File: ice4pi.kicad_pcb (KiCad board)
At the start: 4 copper layers, 65 x 30 mm, 66 parts, among them J1 Pmod 2x6, J2 Raspberry_Pi_2_3, U1 ICE40HX1K-TQ144, U2 W25Q32JVSSIQ(SOIC-8_208mil), U3 LT3030, U4 DSC1001DI1-012.0000, U5 TFDU4101-TR3

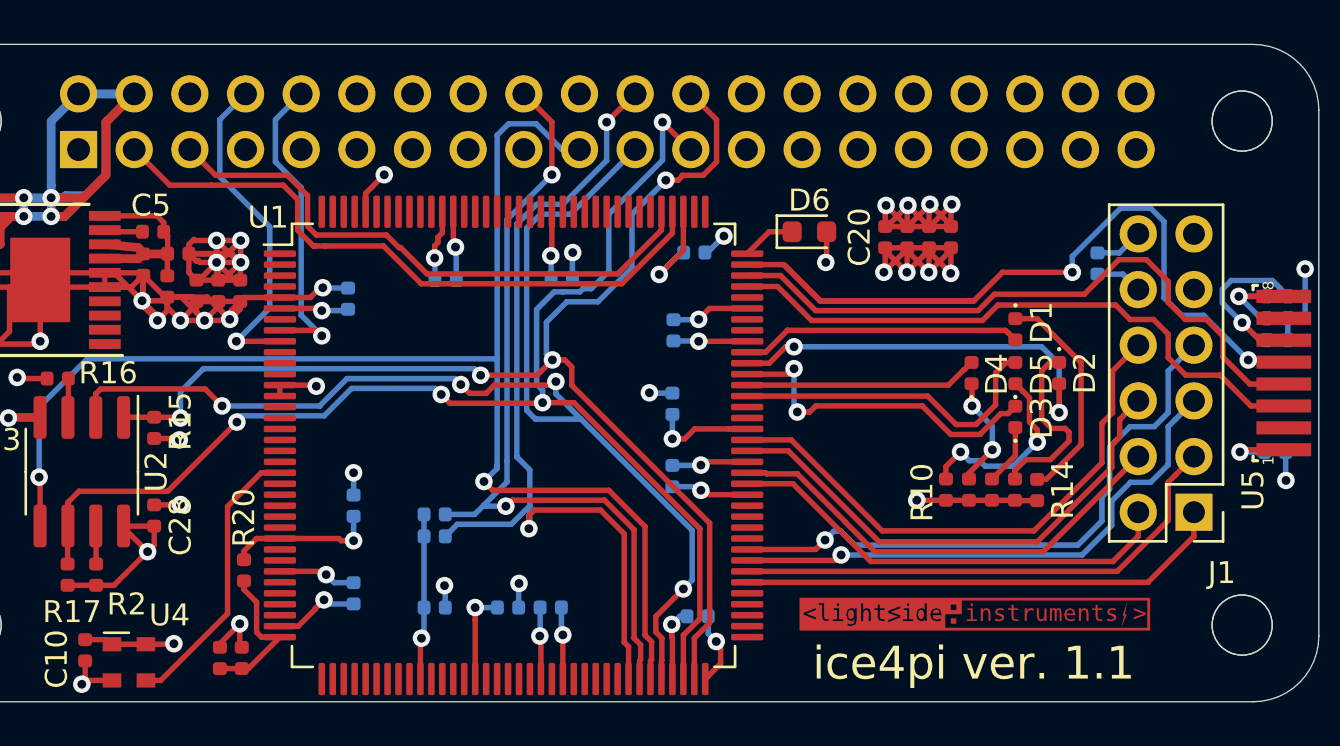
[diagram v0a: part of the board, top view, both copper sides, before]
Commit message: Release 1.2
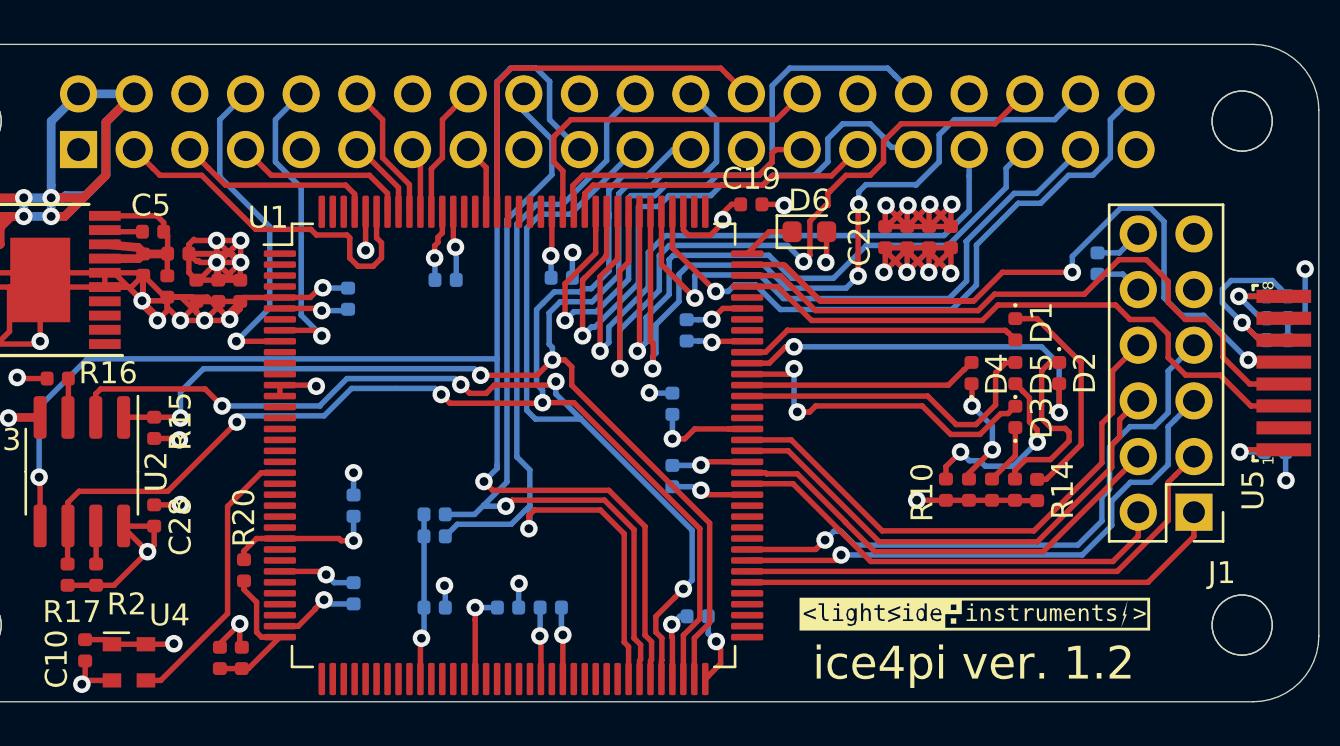
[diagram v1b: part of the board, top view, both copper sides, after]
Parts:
- C19: moved to F.Cu
- U2: value W25Q32JVSSIQ(SOIC-8_208mil) -> W25Q32JVSSIQ
- moved C19 3.41 mm to (89.1, 56.3)
- moved C9 0.60 mm to (86.2, 62.0)
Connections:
- J2 pad 11: Net-(J2-Pad11) -> PIO0_18
- J2 pad 12: Net-(J2-Pad12) -> PIO0_17
- J2 pad 13: Net-(J2-Pad13) -> PIO0_16
- J2 pad 15: Net-(J2-Pad15) -> PIO0_14
- J2 pad 16: Net-(J2-Pad16) -> PIO0_15
- J2 pad 26: Net-(J2-Pad26) -> PIO0_13
- J2 pad 27: Net-(J2-Pad27) -> PIO0_11
- J2 pad 28: Net-(J2-Pad28) -> PIO0_12
- J2 pad 29: Net-(J2-Pad29) -> PIO0_10
- J2 pad 3: PIO0_02 -> PIO0_20
- J2 pad 31: Net-(J2-Pad31) -> PIO0_08
- J2 pad 32: Net-(J2-Pad32) -> PIO0_09
- J2 pad 33: Net-(J2-Pad33) -> PIO0_07
- J2 pad 35: Net-(J2-Pad35) -> PIO0_05
- J2 pad 36: Net-(J2-Pad36) -> PIO0_06
- J2 pad 37: Net-(J2-Pad37) -> PIO0_03
- J2 pad 38: Net-(J2-Pad38) -> PIO0_04
- J2 pad 40: Net-(J2-Pad40) -> PIO0_02
- J2 pad 5: PIO0_03 -> PIO0_21
- J2 pad 7: Net-(J2-Pad7) -> PIO0_19
- U1 pad 120: Net-(U1-Pad120) -> PIO0_10
- U1 pad 121: Net-(U1-Pad121) -> PIO0_11
- U1 pad 122: Net-(U1-Pad122) -> PIO0_12
- U1 pad 128: Net-(U1-Pad128) -> PIO0_13
- U1 pad 129: Net-(U1-Pad129) -> PIO0_14
- U1 pad 134: Net-(U1-Pad134) -> PIO0_15
- U1 pad 135: Net-(U1-Pad135) -> PIO0_16
- U1 pad 136: Net-(U1-Pad136) -> PIO0_17
- U1 pad 137: Net-(U1-Pad137) -> PIO0_18
- U1 pad 138: Net-(U1-Pad138) -> PIO0_19
- U1 pad 139: Net-(U1-Pad139) -> PIO0_20
- U1 pad 141: Net-(U1-Pad141) -> PIO0_21
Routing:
- net PIO0_04: track 0.00 -> 37.6 mm, vias 0 -> 3
- net PIO0_06: track 0.00 -> 35.4 mm, vias 0 -> 2
- net PIO0_09: track 0.00 -> 30.9 mm, vias 0 -> 1
- net PIO0_05: track 0.00 -> 30.9 mm, vias 0 -> 1
- net PIO0_07: track 0.00 -> 30.3 mm, vias 0 -> 1
- net PIO0_08: track 0.00 -> 28.5 mm, vias 0 -> 1
- net PIO0_13: track 0.00 -> 18.0 mm
- net PIO0_20: track 0.00 -> 16.4 mm
- net PIO0_12: track 0.00 -> 15.7 mm
- net PIO0_10: track 0.00 -> 14.1 mm
- net PIO0_11: track 0.00 -> 12.6 mm
- net PIO0_21: track 0.00 -> 9.17 mm
- net PIO0_19: track 0.00 -> 8.15 mm
- net PIO0_17: track 0.00 -> 6.37 mm
- net PIO0_15: track 0.00 -> 6.07 mm
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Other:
- board text added: "ice4pi ver. 1.2"
- board text removed: "ice4pi ver. 1.1"

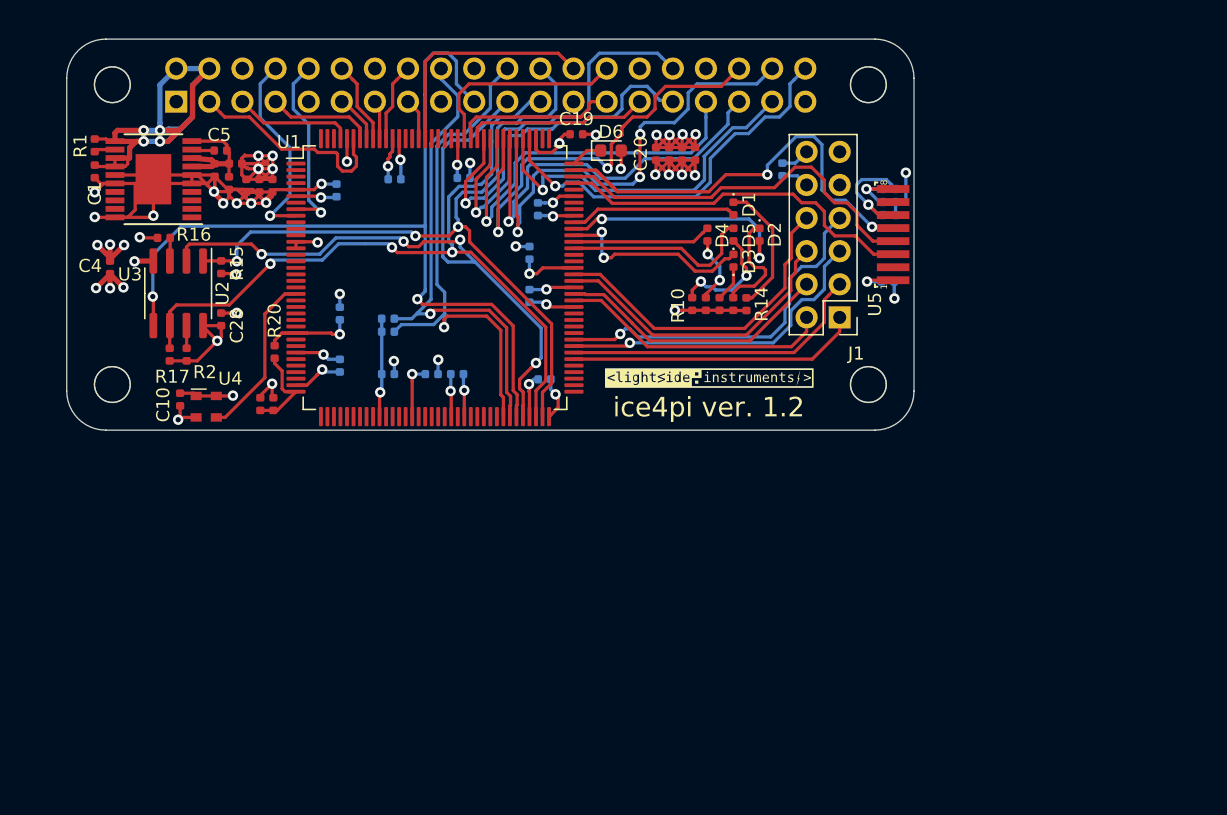
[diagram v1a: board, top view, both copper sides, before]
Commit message: Release ice4pi-gpib-1.0
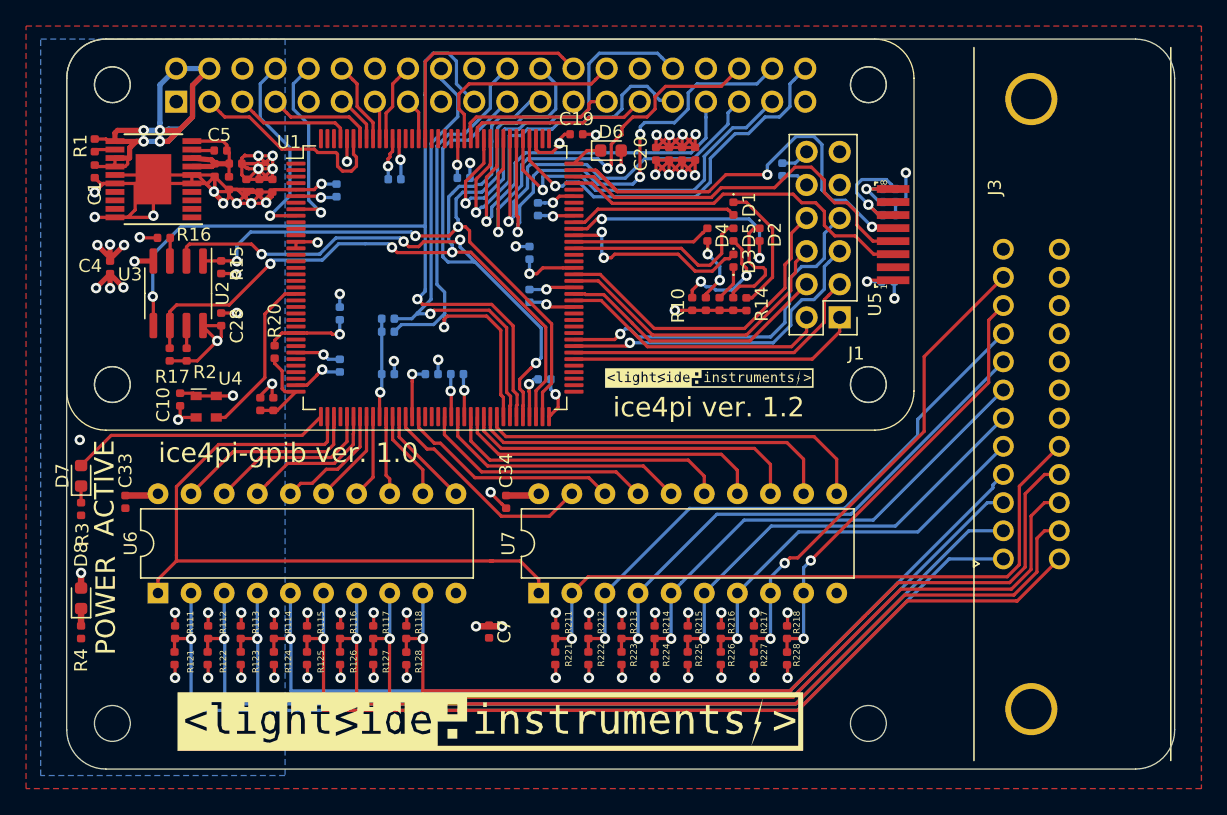
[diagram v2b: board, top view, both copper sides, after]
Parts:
- added ?: , ice4pi:mount_hole, F.Cu at (111.5, 101.5)
- added ?: , ice4pi:mount_hole, F.Cu at (53.5, 101.5)
- added C33: 220 nF, Capacitor_SMD:C_0402_1005Metric, F.Cu at (54.5, 84.5)
- added C34: 220 nF, Capacitor_SMD:C_0402_1005Metric, F.Cu at (83.7, 84.5)
- added C7: 10 uF, Capacitor_SMD:C_0402_1005Metric, F.Cu at (82.4, 94.5)
- added D7: LED, LED_SMD:LED_0603_1608Metric, F.Cu at (51.1, 82.5)
- added D8: LED, LED_SMD:LED_0603_1608Metric, F.Cu at (51.1, 91.9)
- added J3: Conn_02x12_Top_Bottom, ice4pi:centronix-24-male, F.Cu at (124.0, 77.0)
- added R111: 3K, Resistor_SMD:R_0402_1005Metric, F.Cu at (58.3, 94.5)
- added R112: 3K, Resistor_SMD:R_0402_1005Metric, F.Cu at (60.9, 94.5)
- added R113: 3K, Resistor_SMD:R_0402_1005Metric, F.Cu at (63.4, 94.5)
- added R114: 3K, Resistor_SMD:R_0402_1005Metric, F.Cu at (65.9, 94.5)
- added R115: 3K, Resistor_SMD:R_0402_1005Metric, F.Cu at (68.4, 94.5)
- added R116: 3K, Resistor_SMD:R_0402_1005Metric, F.Cu at (71.0, 94.5)
- added R117: 3.3K, Resistor_SMD:R_0402_1005Metric, F.Cu at (73.5, 94.5)
- added R118: 3K, Resistor_SMD:R_0402_1005Metric, F.Cu at (76.0, 94.5)
- added R121: 6.2K, Resistor_SMD:R_0402_1005Metric, F.Cu at (58.3, 96.5)
- added R122: 6.2K, Resistor_SMD:R_0402_1005Metric, F.Cu at (60.8, 96.5)
- added R123: 6.2K, Resistor_SMD:R_0402_1005Metric, F.Cu at (63.4, 96.5)
- added R124: 6.2K, Resistor_SMD:R_0402_1005Metric, F.Cu at (65.9, 96.5)
- added R125: 6.2K, Resistor_SMD:R_0402_1005Metric, F.Cu at (68.4, 96.5)
- added R126: 6.2K, Resistor_SMD:R_0402_1005Metric, F.Cu at (71.0, 96.5)
- added R127: 6.2K, Resistor_SMD:R_0402_1005Metric, F.Cu at (73.5, 96.5)
- added R128: 6.2K, Resistor_SMD:R_0402_1005Metric, F.Cu at (76.0, 96.5)
- added R211: 3K, Resistor_SMD:R_0402_1005Metric, F.Cu at (87.5, 94.5)
- added R212: 3K, Resistor_SMD:R_0402_1005Metric, F.Cu at (90.0, 94.5)
- added R213: 3K, Resistor_SMD:R_0402_1005Metric, F.Cu at (92.6, 94.5)
- added R214: 3K, Resistor_SMD:R_0402_1005Metric, F.Cu at (95.1, 94.5)
- added R215: 3K, Resistor_SMD:R_0402_1005Metric, F.Cu at (97.6, 94.5)
- added R216: 3K, Resistor_SMD:R_0402_1005Metric, F.Cu at (100.2, 94.5)
- added R217: 3.3K, Resistor_SMD:R_0402_1005Metric, F.Cu at (102.7, 94.5)
- added R218: 3K, Resistor_SMD:R_0402_1005Metric, F.Cu at (105.3, 94.5)
- added R221: 6.2K, Resistor_SMD:R_0402_1005Metric, F.Cu at (87.5, 96.5)
- added R222: 6.2K, Resistor_SMD:R_0402_1005Metric, F.Cu at (90.0, 96.5)
- added R223: 6.2K, Resistor_SMD:R_0402_1005Metric, F.Cu at (92.6, 96.5)
- added R224: 6.2K, Resistor_SMD:R_0402_1005Metric, F.Cu at (95.1, 96.5)
- added R225: 6.2K, Resistor_SMD:R_0402_1005Metric, F.Cu at (97.6, 96.5)
- added R226: 6.2K, Resistor_SMD:R_0402_1005Metric, F.Cu at (100.2, 96.5)
- added R227: 6.2K, Resistor_SMD:R_0402_1005Metric, F.Cu at (102.7, 96.5)
- added R228: 6.2K, Resistor_SMD:R_0402_1005Metric, F.Cu at (105.3, 96.5)
- added R3: 1K, Resistor_SMD:R_0402_1005Metric, F.Cu at (51.1, 85.0)
- added R4: 1K, Resistor_SMD:R_0402_1005Metric, F.Cu at (51.1, 94.5)
- added U6: SN75160BN, Package_DIP:DIP-20_W7.62mm, F.Cu at (57.0, 91.5)
- added U7: SN75161BN, Package_DIP:DIP-20_W7.62mm, F.Cu at (86.2, 91.5)
- added svg2mod: G***, ice4pi:lsi-logo-48mm, F.Cu at (82.5, 103.0)
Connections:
- U1 pad 1: Net-(U1-Pad1) -> (no net)
- U1 pad 10: Net-(U1-Pad10) -> (no net)
- U1 pad 101: Net-(U1-Pad101) -> (no net)
- U1 pad 102: Net-(U1-Pad102) -> (no net)
- U1 pad 104: Net-(U1-Pad104) -> (no net)
- U1 pad 109: Net-(U1-Pad109) -> (no net)
- U1 pad 11: Net-(U1-Pad11) -> (no net)
- U1 pad 110: Net-(U1-Pad110) -> (no net)
- U1 pad 12: Net-(U1-Pad12) -> (no net)
- U1 pad 124: Net-(U1-Pad124) -> (no net)
- U1 pad 125: Net-(U1-Pad125) -> (no net)
- U1 pad 126: Net-(U1-Pad126) -> (no net)
- U1 pad 127: Net-(U1-Pad127) -> (no net)
- U1 pad 130: Net-(U1-Pad130) -> (no net)
- U1 pad 131: Net-(U1-Pad131) -> (no net)
- U1 pad 142: Net-(U1-Pad142) -> (no net)
- U1 pad 143: Net-(U1-Pad143) -> (no net)
- U1 pad 144: Net-(U1-Pad144) -> (no net)
- U1 pad 15: Net-(U1-Pad15) -> (no net)
- U1 pad 16: Net-(U1-Pad16) -> (no net)
- U1 pad 17: Net-(U1-Pad17) -> (no net)
- U1 pad 18: Net-(U1-Pad18) -> (no net)
- U1 pad 19: Net-(U1-Pad19) -> (no net)
- U1 pad 2: Net-(U1-Pad2) -> (no net)
- U1 pad 20: Net-(U1-Pad20) -> (no net)
- U1 pad 22: Net-(U1-Pad22) -> (no net)
- U1 pad 23: Net-(U1-Pad23) -> (no net)
- U1 pad 24: Net-(U1-Pad24) -> (no net)
- U1 pad 25: Net-(U1-Pad25) -> (no net)
- U1 pad 26: Net-(U1-Pad26) -> (no net)
- U1 pad 28: Net-(U1-Pad28) -> (no net)
- U1 pad 29: Net-(U1-Pad29) -> (no net)
- U1 pad 3: Net-(U1-Pad3) -> (no net)
- U1 pad 31: Net-(U1-Pad31) -> (no net)
- U1 pad 32: Net-(U1-Pad32) -> (no net)
- U1 pad 33: Net-(U1-Pad33) -> (no net)
- U1 pad 34: Net-(U1-Pad34) -> (no net)
- U1 pad 37: Net-(U1-Pad37) -> /CTRL_LED
- U1 pad 38: Net-(U1-Pad38) -> /GPIB_TE
- U1 pad 39: Net-(U1-Pad39) -> /GPIB_DIO01
- U1 pad 4: Net-(U1-Pad4) -> (no net)
- U1 pad 40: Net-(U1-Pad40) -> (no net)
- U1 pad 41: Net-(U1-Pad41) -> /GPIB_DIO02
- U1 pad 42: Net-(U1-Pad42) -> /GPIB_DIO03
- U1 pad 43: Net-(U1-Pad43) -> /GPIB_DIO04
- U1 pad 44: Net-(U1-Pad44) -> /GPIB_DIO05
- U1 pad 45: Net-(U1-Pad45) -> /GPIB_DIO06
- U1 pad 47: Net-(U1-Pad47) -> /GPIB_DIO07
- U1 pad 48: Net-(U1-Pad48) -> /GPIB_DIO08
- U1 pad 49: Net-(U1-Pad49) -> /GPIB_PE
- U1 pad 50: Net-(U1-Pad50) -> /GPIB_REN
- U1 pad 52: Net-(U1-Pad52) -> /GPIB_IFC
- U1 pad 53: Net-(U1-Pad53) -> (no net)
- U1 pad 54: Net-(U1-Pad54) -> (no net)
- U1 pad 55: Net-(U1-Pad55) -> (no net)
- U1 pad 56: Net-(U1-Pad56) -> /GPIB_NDAC
- U1 pad 58: Net-(U1-Pad58) -> /GPIB_NRFD
- U1 pad 60: Net-(U1-Pad60) -> /GPIB_DAV
- U1 pad 61: Net-(U1-Pad61) -> /GPIB_EOI
- U1 pad 62: Net-(U1-Pad62) -> /GPIB_ATN
- U1 pad 63: Net-(U1-Pad63) -> /GPIB_SRQ
- U1 pad 64: Net-(U1-Pad64) -> /GPIB_DC
- U1 pad 7: Net-(U1-Pad7) -> (no net)
- U1 pad 73: Net-(U1-Pad73) -> (no net)
- U1 pad 74: Net-(U1-Pad74) -> (no net)
- U1 pad 75: Net-(U1-Pad75) -> (no net)
- U1 pad 76: Net-(U1-Pad76) -> (no net)
- U1 pad 77: Net-(U1-Pad77) -> (no net)
- U1 pad 82: Net-(U1-Pad82) -> (no net)
- U1 pad 83: Net-(U1-Pad83) -> (no net)
- U1 pad 84: Net-(U1-Pad84) -> (no net)
- U1 pad 85: Net-(U1-Pad85) -> (no net)
- U1 pad 93: Net-(U1-Pad93) -> (no net)
- U1 pad 94: Net-(U1-Pad94) -> (no net)
- U3 pad 1: Net-(U3-Pad1) -> (no net)
- U3 pad 17: Net-(U3-Pad17) -> (no net)
- U3 pad 18: Net-(U3-Pad18) -> (no net)
- U3 pad 19: Net-(U3-Pad19) -> (no net)
- U3 pad 2: Net-(U3-Pad2) -> (no net)
- U3 pad 3: Net-(U3-Pad3) -> (no net)
- U3 pad 4: Net-(U3-Pad4) -> (no net)
- U5 pad 2: Net-(U5-Pad2) -> (no net)
- U5 pad 7: Net-(U5-Pad7) -> (no net)
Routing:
- net /DIO01: track 0.00 -> 78.6 mm, vias 0 -> 1
- net /DIO02: track 0.00 -> 76.0 mm, vias 0 -> 1
- net /DIO03: track 0.00 -> 73.7 mm, vias 0 -> 1
- net /DIO05: track 0.00 -> 72.6 mm, vias 0 -> 1
- net /DIO04: track 0.00 -> 71.7 mm, vias 0 -> 1
- net /DIO06: track 0.00 -> 71.7 mm, vias 0 -> 1
- net /DIO07: track 0.00 -> 70.3 mm, vias 0 -> 1
- net /DIO08: track 0.00 -> 69.0 mm, vias 0 -> 1
- net /GPIB_TE: track 0.00 -> 53.3 mm
- net /REN: track 0.00 -> 51.4 mm, vias 0 -> 1
- net /IFC: track 0.00 -> 45.3 mm, vias 0 -> 1
- net /NDAC: track 0.00 -> 41.2 mm, vias 0 -> 1
- net /ATN: track 0.00 -> 37.8 mm, vias 0 -> 2
- net /NRFD: track 0.00 -> 37.7 mm, vias 0 -> 1
- net /DAV: track 0.00 -> 34.3 mm, vias 0 -> 1
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- added copper zone on B.Cu, net +5V
- added copper zone on In2.Cu, net +5V
- added copper zone on F.Cu, net GND
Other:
- board size 65 x 30 mm -> 85 x 56 mm
- board text added: "ACTIVE"
- board text added: "POWER"
- board text added: "ice4pi-gpib ver. 1.0"
